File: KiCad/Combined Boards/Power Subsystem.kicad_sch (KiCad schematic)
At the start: 26 parts, among them J1 Solar Panel, J2 Charge Status, J4 Battery, J5 3.3V, Q1 SI2301CDS-T1-GE3, U2 XC6210B332MR

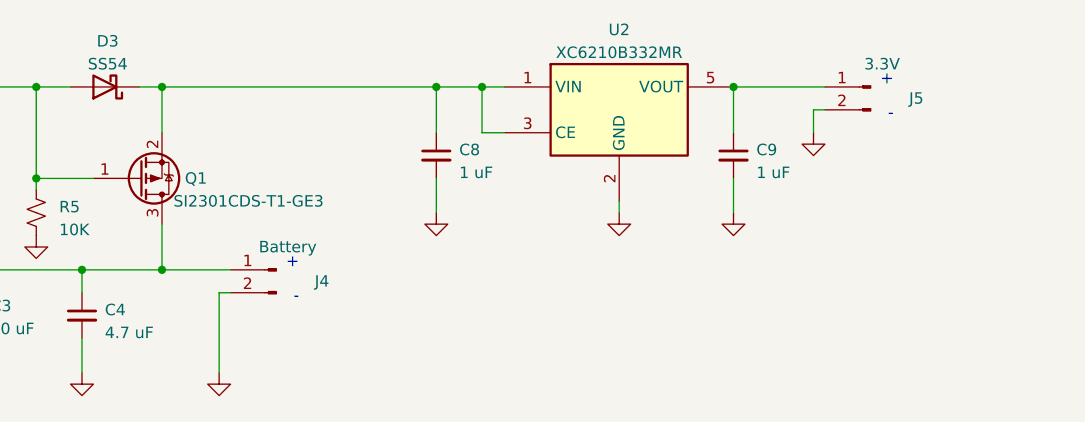
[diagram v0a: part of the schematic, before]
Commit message: More work on power subsystem
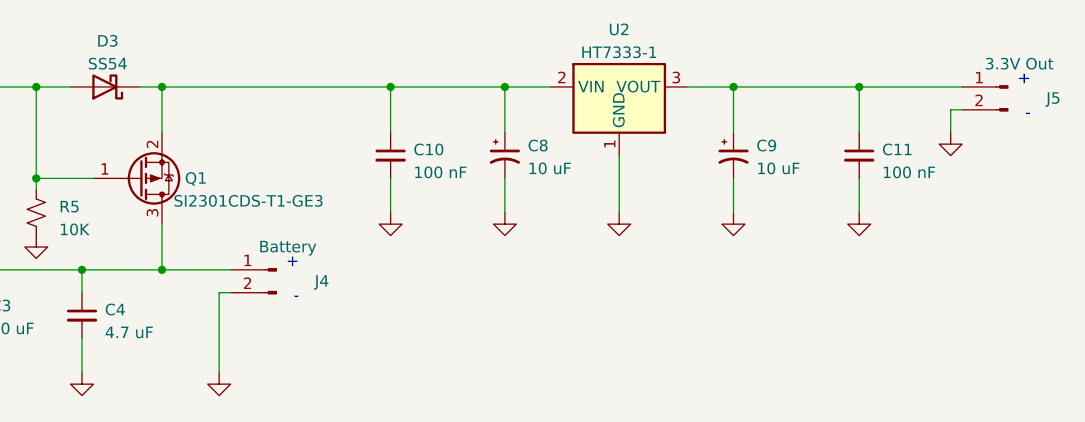
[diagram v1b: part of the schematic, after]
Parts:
- removed C8, C9: 1 uF, symbol Device:C_Small
- removed U2: XC6210B332MR, Package_TO_SOT_SMD:SOT-23-5, symbol Regulator_Linear:XC6210B332MR
- added C10, C11: 100 nF, symbol Device:C_Small
- added C8, C9: 10 uF, symbol Device:C_Polarized_Small_US
- added U2: HT7333-1, Package_TO_SOT_SMD:SOT-89-3, symbol Regulator_Linear:HT75xx-1-SOT89
- J5: value 3.3V -> 3.3V Out
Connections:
- net GND: now also C10.2, C11.2, C8.2, C9.2, U2.1 (GND)
- net at J5.1 (Pin_1): now also C11.1, C9.1, U2.3 (VOUT)
- net at D3.1 (K), Q1.2 (S): now also C10.1, C8.1, U2.2 (VIN)
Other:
- moved on the sheet: J5
